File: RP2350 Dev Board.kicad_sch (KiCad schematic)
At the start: 62 parts, among them J1 Conn_01x32_MountingPin, J2 Conn_01x03_Pin, J3 Conn_01x32_MountingPin, U4 Winbond W25Q128JVSIQ, U5 RPI Radio Module 2, U6 ESP-PSRAM32

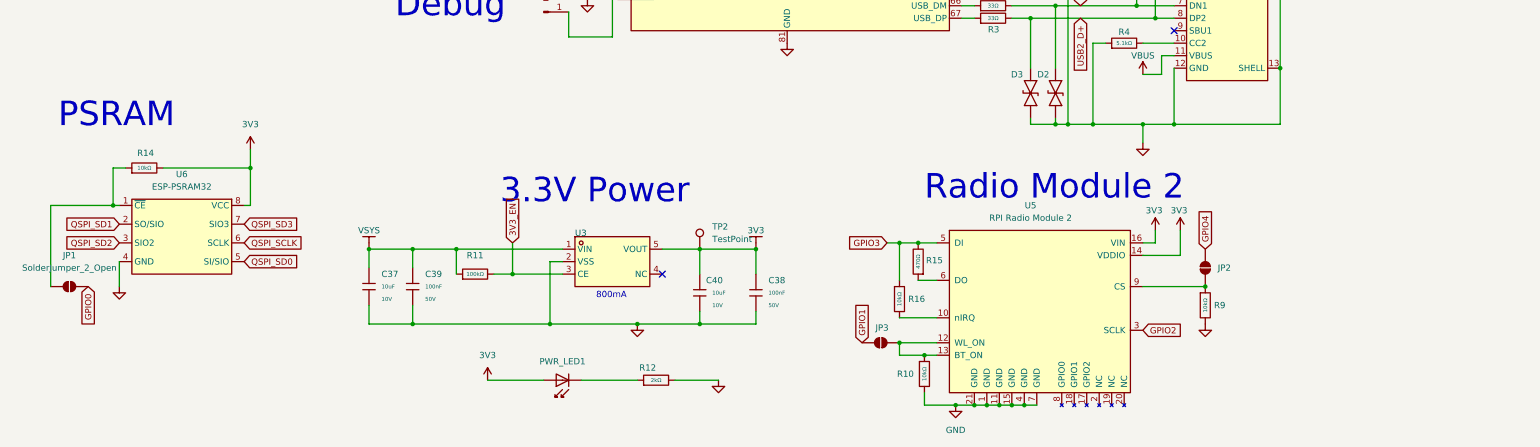
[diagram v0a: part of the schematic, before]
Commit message: Cleanup
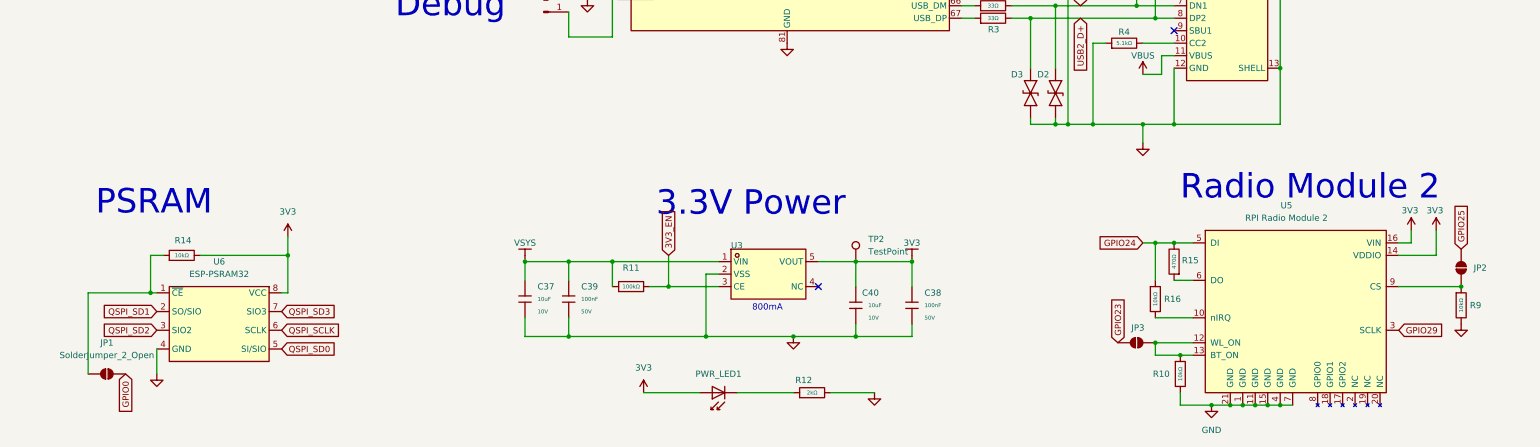
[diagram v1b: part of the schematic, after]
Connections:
- net GPIO1: no longer JP3.1 (A)
- net GPIO2: no longer U5.3 (SCLK)
- net GPIO23: now also JP3.1 (A)
- net GPIO24: now also R15.2, R16.1, U5.5 (DI)
- net GPIO25: now also JP2.2 (B)
- net GPIO29: now also U5.3 (SCLK)
- net GPIO3: no longer R15.2, R16.1, U5.5 (DI)
- net GPIO4: no longer JP2.2 (B)
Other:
- moved on the sheet: C37, C38, C39, C40, JP1, JP2, JP3, PWR_LED1, R10, R11, R12, R14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
